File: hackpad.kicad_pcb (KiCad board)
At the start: 2 copper layers, 19 x 57 mm, 4 parts, among them SW1 SW_Push, SW2 SW_Push, SW3 SW_Push, U1 MOUDLE-SEEEDUINO-XIAO

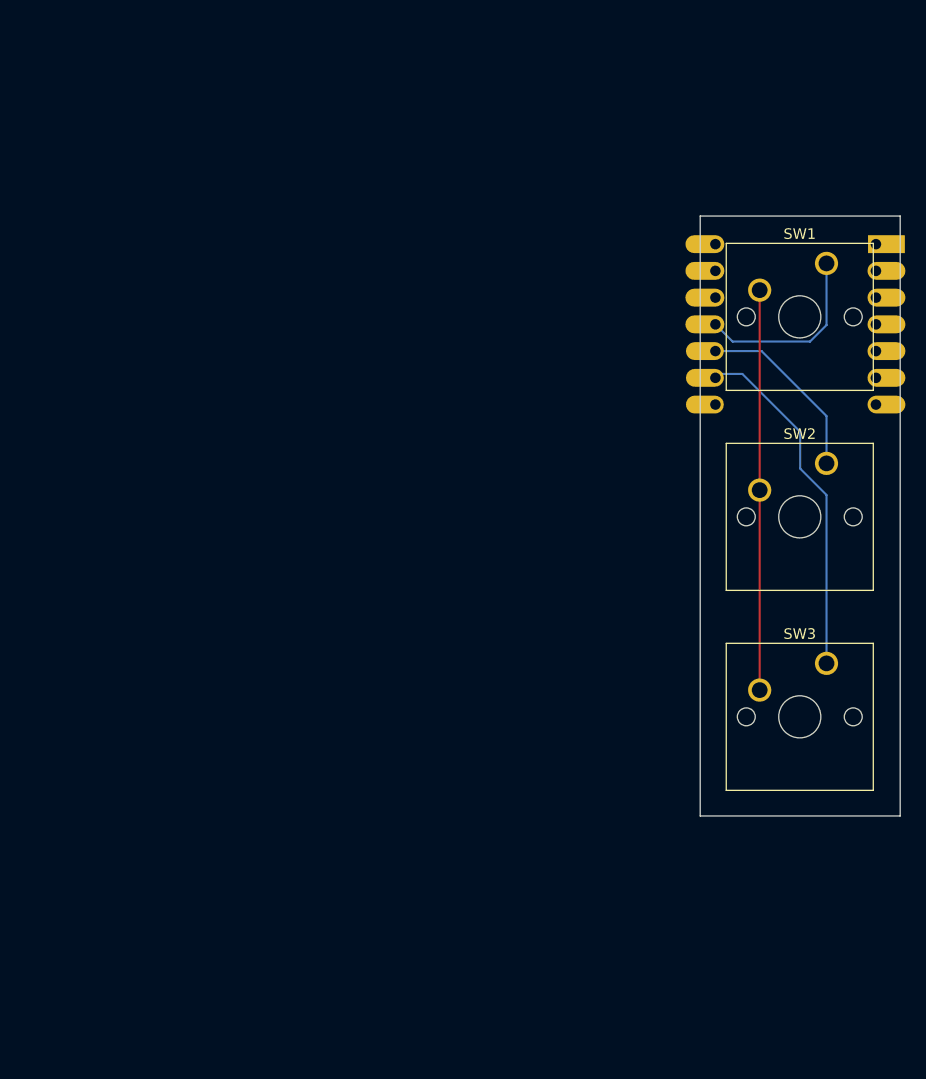
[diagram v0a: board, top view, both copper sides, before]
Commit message: Add files via upload
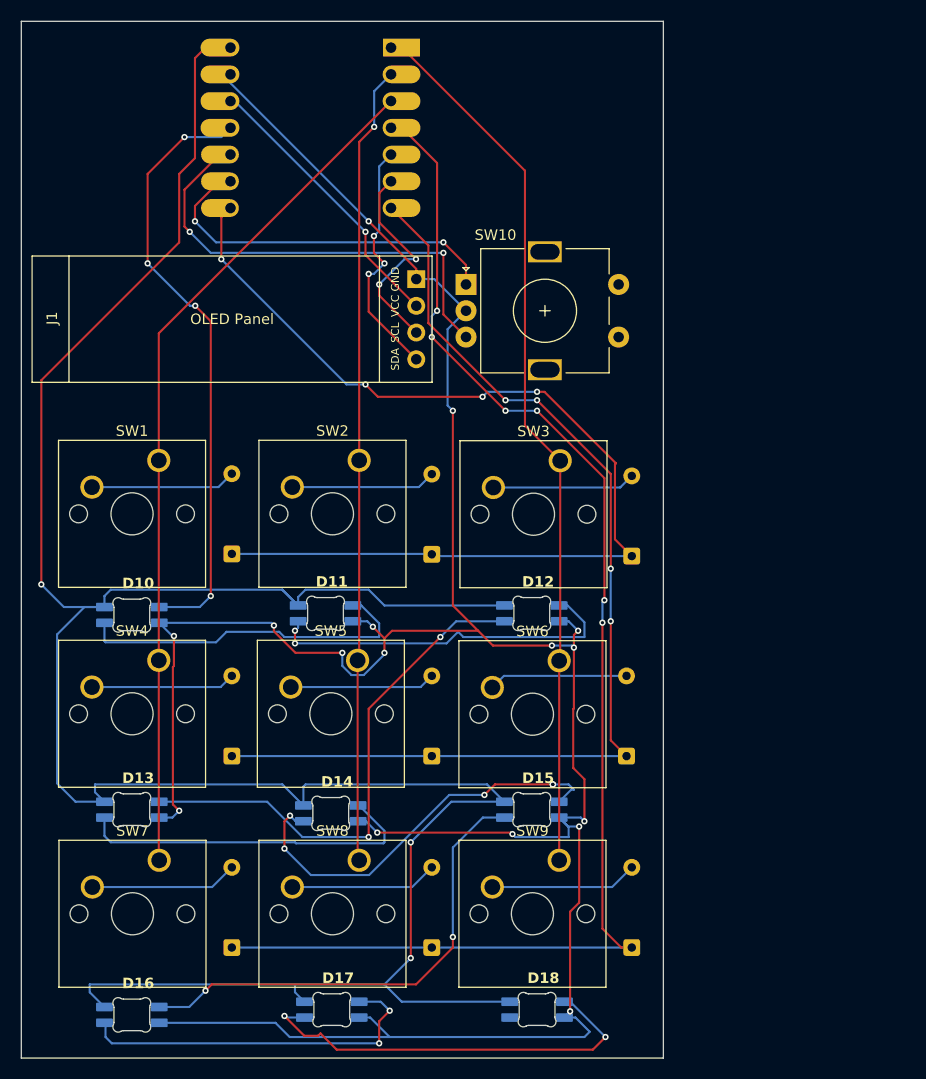
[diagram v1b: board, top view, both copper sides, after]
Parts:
- added D1: ~, Diode_THT:D_DO-35_SOD27_P7.62mm_Horizontal, B.Cu at (76.5, 116.1)
- added D10: SK6812MINI-E, footprints:SK6812MINI-E_fixed, F.Cu at (67.0, 122.0)
- added D11: SK6812MINI-E, footprints:SK6812MINI-E_fixed, F.Cu at (85.4, 121.9)
- added D12: SK6812MINI-E, footprints:SK6812MINI-E_fixed, F.Cu at (105.0, 121.9)
- added D13: SK6812MINI-E, footprints:SK6812MINI-E_fixed, F.Cu at (67.0, 140.5)
- added D14: SK6812MINI-E, footprints:SK6812MINI-E_fixed, F.Cu at (85.9, 140.9)
- added D15: SK6812MINI-E, footprints:SK6812MINI-E_fixed, F.Cu at (105.0, 140.5)
- added D16: SK6812MINI-E, footprints:SK6812MINI-E_fixed, F.Cu at (67.0, 160.0)
- added D17: SK6812MINI-E, footprints:SK6812MINI-E_fixed, F.Cu at (86.0, 159.5)
- added D18: SK6812MINI-E, footprints:SK6812MINI-E_fixed, F.Cu at (105.5, 159.5)
- added D2: ~, Diode_THT:D_DO-35_SOD27_P7.62mm_Horizontal, B.Cu at (95.5, 116.1)
- added D3: ~, Diode_THT:D_DO-35_SOD27_P7.62mm_Horizontal, B.Cu at (114.5, 116.3)
- added D4: ~, Diode_THT:D_DO-35_SOD27_P7.62mm_Horizontal, B.Cu at (76.5, 135.3)
- added D5: ~, Diode_THT:D_DO-35_SOD27_P7.62mm_Horizontal, B.Cu at (95.5, 135.3)
- added D6: ~, Diode_THT:D_DO-35_SOD27_P7.62mm_Horizontal, B.Cu at (114.0, 135.3)
- added D7: ~, Diode_THT:D_DO-35_SOD27_P7.62mm_Horizontal, B.Cu at (76.5, 153.5)
- added D8: ~, Diode_THT:D_DO-35_SOD27_P7.62mm_Horizontal, B.Cu at (95.5, 153.5)
- added D9: ~, Diode_THT:D_DO-35_SOD27_P7.62mm_Horizontal, B.Cu at (114.5, 153.5)
- added J1: OLED_128x32, KiCad-SSD1306-0.91-OLED-4pin-128x32.pretty-master:SSD1306-0.91-OLED-4pin-128x32, F.Cu at (57.5, 87.8)
- added SW10: RotaryEncoder_Switch, Rotary_Encoder:RotaryEncoder_Alps_EC11E-Switch_Vertical_H20mm, F.Cu at (98.8, 90.5)
- added SW4: SW_Push, Button_Switch_Keyboard:SW_Cherry_MX_1.00u_PCB, F.Cu at (69.6, 126.2)
- added SW5: SW_Push, Button_Switch_Keyboard:SW_Cherry_MX_1.00u_PCB, F.Cu at (88.5, 126.2)
- added SW6: SW_Push, Button_Switch_Keyboard:SW_Cherry_MX_1.00u_PCB, F.Cu at (107.6, 126.2)
- added SW7: SW_Push, Button_Switch_Keyboard:SW_Cherry_MX_1.00u_PCB, F.Cu at (69.6, 145.2)
- added SW8: SW_Push, Button_Switch_Keyboard:SW_Cherry_MX_1.00u_PCB, F.Cu at (88.6, 145.2)
- added SW9: SW_Push, Button_Switch_Keyboard:SW_Cherry_MX_1.00u_PCB, F.Cu at (107.6, 145.2)
- moved SW1 66.1 mm to (69.6, 107.2)
- moved U1 49.7 mm to (84.0, 75.6)
- moved SW2 44.4 mm to (88.6, 107.2)
- moved SW3 31.8 mm to (107.7, 107.2)
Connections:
- SW1 pad 1: Net-(U1-PA6_A10_D10_MOSI) -> Column 1
- SW1 pad 2: GND -> Net-(D1-A)
- SW2 pad 1: Net-(U1-PA5_A9_D9_MISO) -> Column 2
- SW2 pad 2: GND -> Net-(D2-A)
- SW3 pad 1: Net-(U1-PA7_A8_D8_SCK) -> Column 3
- SW3 pad 2: GND -> Net-(D3-A)
- U1 pad 1: unconnected-(U1-PA02_A0_D0-Pad1) -> Column 3
- U1 pad 10: Net-(U1-PA5_A9_D9_MISO) -> Rotary B
- U1 pad 11: Net-(U1-PA6_A10_D10_MOSI) -> rgbdata
- U1 pad 12: unconnected-(U1-3V3-Pad12) -> +3.3V
- U1 pad 14: unconnected-(U1-5V-Pad14) -> +5V
- U1 pad 2: unconnected-(U1-PA4_A1_D1-Pad2) -> Column 2
- U1 pad 3: unconnected-(U1-PA10_A2_D2-Pad3) -> Column 1
- U1 pad 4: unconnected-(U1-PA11_A3_D3-Pad4) -> Row 3
- U1 pad 5: unconnected-(U1-PA8_A4_D4_SDA-Pad5) -> oled sda
- U1 pad 6: unconnected-(U1-PA9_A5_D5_SCL-Pad6) -> oled scl
- U1 pad 7: unconnected-(U1-PB08_A6_D6_TX-Pad7) -> Row 2
- U1 pad 8: unconnected-(U1-PB09_A7_D7_RX-Pad8) -> Row 1
- U1 pad 9: Net-(U1-PA7_A8_D8_SCK) -> Rotary A
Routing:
- net +5V: track 0.00 -> 250.1 mm, vias 0 -> 3
- net GND: track 38.0 -> 251.1 mm, vias 0 -> 16
- net Row 3: track 0.00 -> 128.9 mm, vias 0 -> 6
- net Row 2: track 0.00 -> 100.6 mm, vias 0 -> 4
- net Row 1: track 0.00 -> 98.8 mm, vias 0 -> 4
- net Column 3: track 0.00 -> 84.5 mm
- net Column 1: track 0.00 -> 81.3 mm
- net Column 2: track 0.00 -> 76.0 mm, vias 0 -> 1
- net rgbdata: track 0.00 -> 57.9 mm, vias 0 -> 4
- net Net-(D12-DOUT): track 0.00 -> 49.8 mm, vias 0 -> 2
- net Net-(D15-DOUT): track 0.00 -> 45.8 mm, vias 0 -> 2
- net Rotary B: track 0.00 -> 43.8 mm, vias 0 -> 2
- net Net-(D17-DOUT): track 0.00 -> 39.8 mm, vias 0 -> 2
- net Net-(D14-DOUT): track 0.00 -> 39.2 mm, vias 0 -> 5
- net Rotary A: track 0.00 -> 35.1 mm, vias 0 -> 2
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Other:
- board size 19 x 57 mm -> 61 x 98.5 mm
